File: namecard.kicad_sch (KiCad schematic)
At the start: 37 parts, among them J1 Conn_01x24, J2 Conn_01x05, Q1 AO3400A, U1 STM32G030K6Tx, U2 ST25DV04K-IER8C3

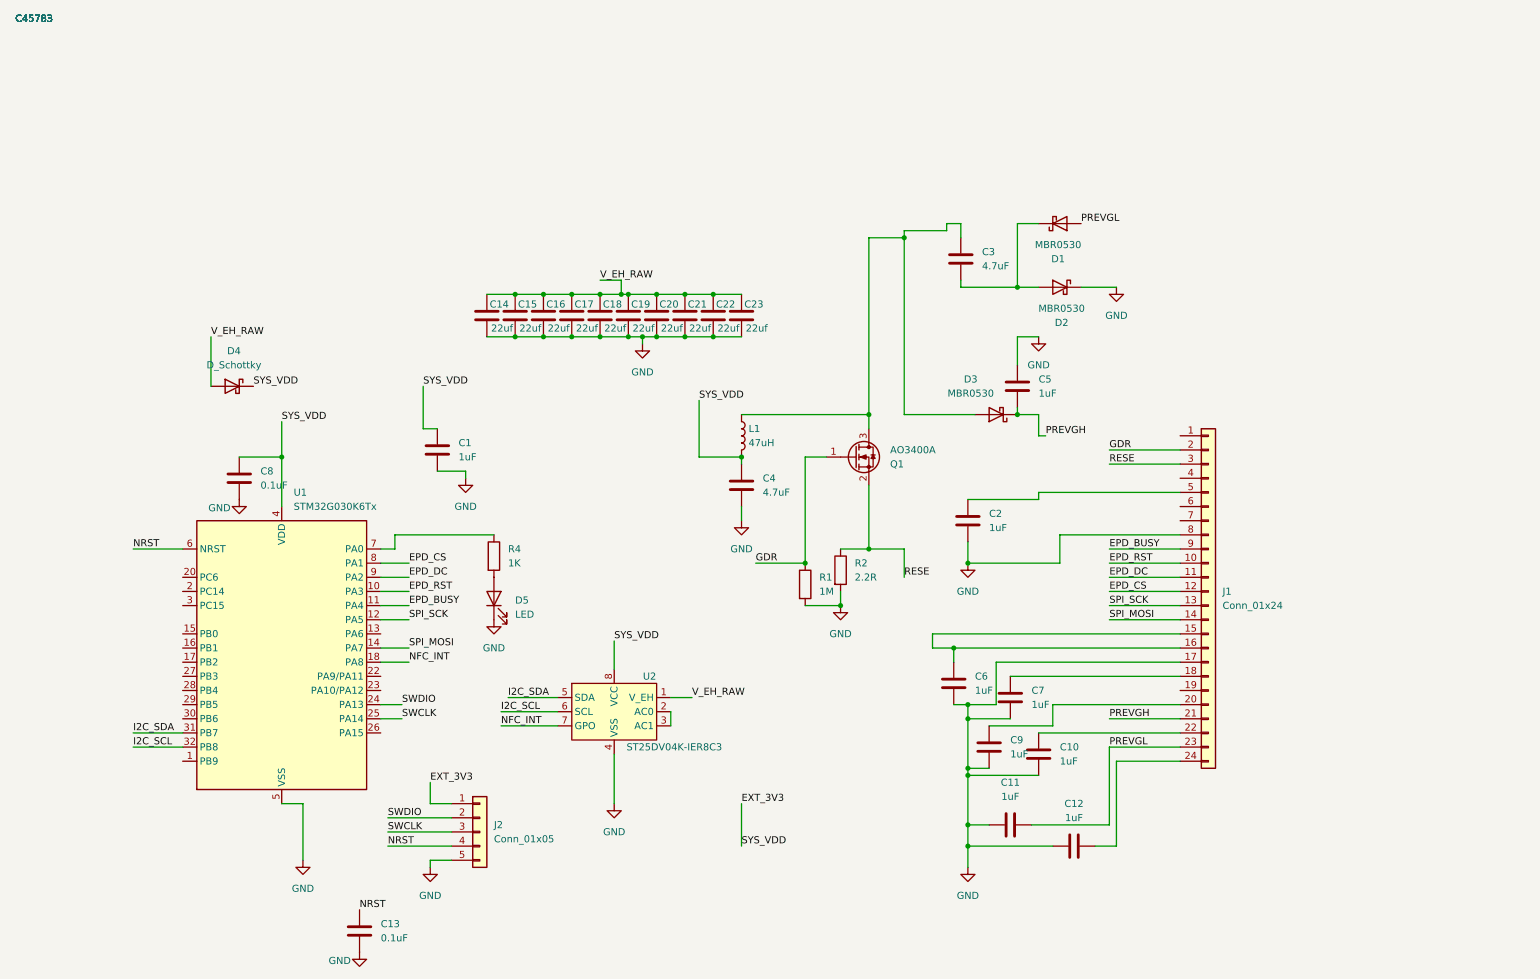
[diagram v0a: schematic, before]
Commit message: v3
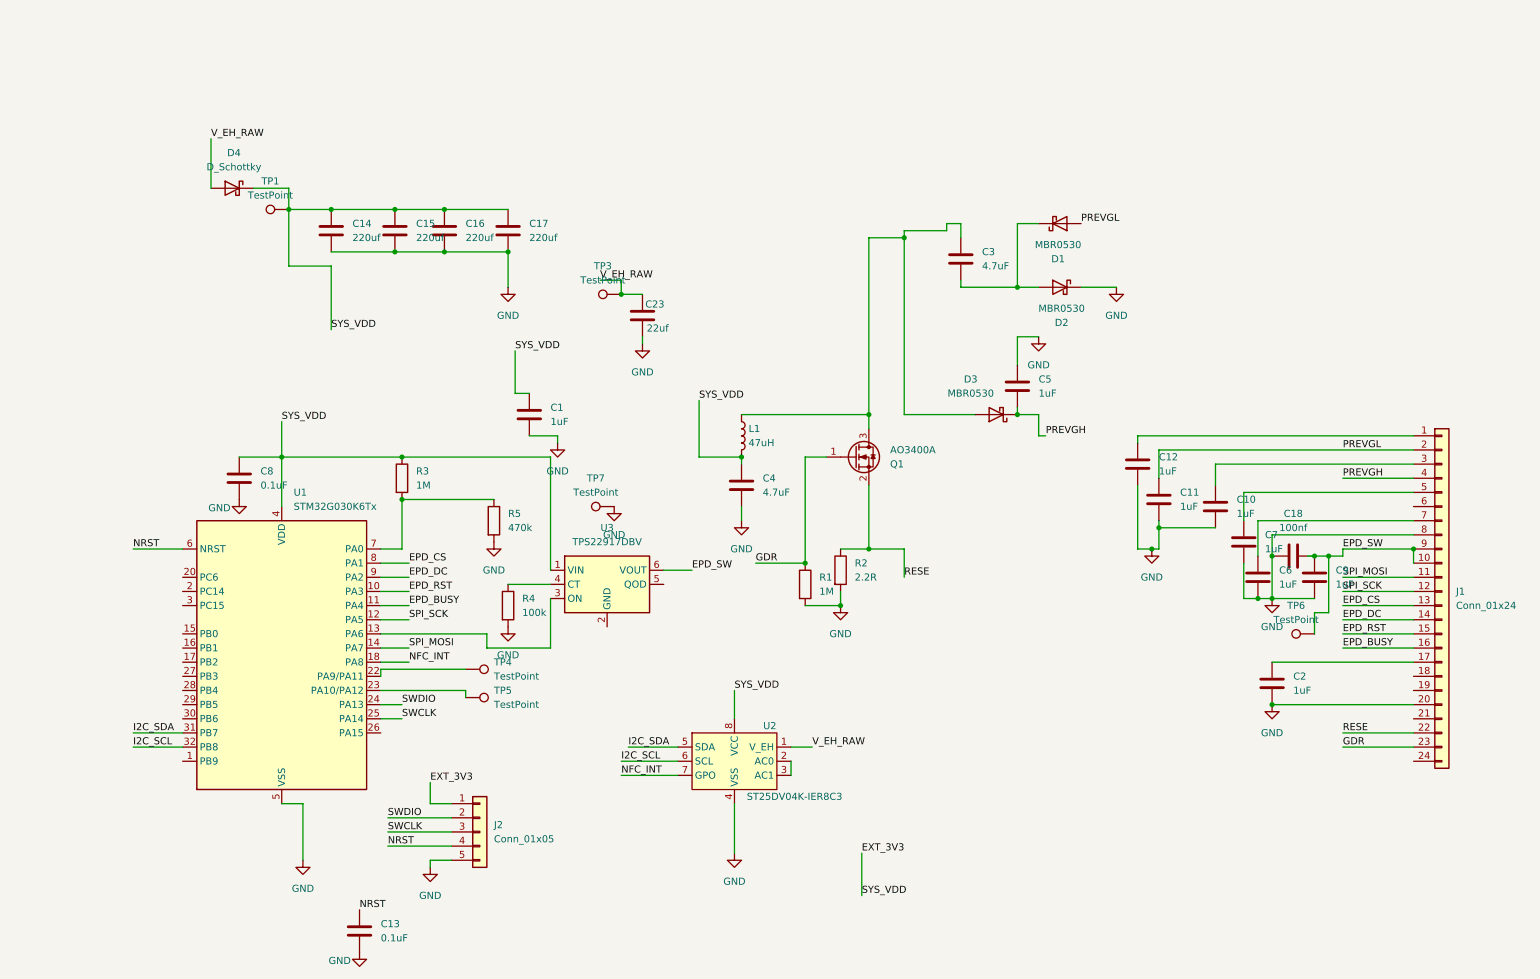
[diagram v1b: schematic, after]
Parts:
- removed C19, C20, C21, C22: 22uf, Capacitor_SMD:C_0805_2012Metric, symbol Device:C
- removed D5: LED, LED_SMD:LED_0603_1608Metric, symbol Device:LED
- added R3: 1M, Resistor_SMD:R_0603_1608Metric, symbol Device:R
- added R5: 470k, Resistor_SMD:R_0603_1608Metric, symbol Device:R
- added TP1, TP3, TP4, TP5, TP6, TP7: TestPoint, TestPoint:TestPoint_Pad_D1.0mm, symbol Connector:TestPoint
- added U3: TPS22917DBV, Package_TO_SOT_SMD:SOT-23-6, symbol Power_Management:TPS22917DBV
- C14, C15, C16, C17: value 22uf -> 220uf; footprint Capacitor_SMD:C_0805_2012Metric -> Capacitor_Tantalum_SMD:6TPE220MAZB; JLCPCB (none) -> C79111; LCSC C45783 -> (none)
- C18: value 22uf -> 100nf; footprint Capacitor_SMD:C_0805_2012Metric -> Capacitor_SMD:C_0603_1608Metric; LCSC C45783 -> (none)
- C23: JLCPCB (none) -> C45783; LCSC C45783 -> (none)
- D4: footprint Diode_SMD:D_SOD-123 -> Diode_SMD:D_SOD-123F; JLCPCB (none) -> C110921; LCSC C22374920 -> (none)
- J1: footprint Connector:FFC-SMD_24P-P0.50_FH34SRJ-24S-0.5SH -> Connector_FFC-FPC:Hirose_FH12-24S-0.5SH_1x24-1MP_P0.50mm_Horizontal; JLCPCB (none) -> C506794; LCSC C324726 -> (none)
- L1: JLCPCB (none) -> C66936; LCSC C66936 -> (none)
- R4: value 1K -> 100k
- U1: JLCPCB (none) -> C529331; LCSC C529331 -> (none)
- U2: JLCPCB (none) -> C2908287; LCSC C2908287 -> (none)
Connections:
- net EPD_BUSY: now also J1.16 (Pin_16); no longer J1.9 (Pin_9)
- net EPD_CS: now also J1.13 (Pin_13); no longer J1.12 (Pin_12)
- net EPD_DC: now also J1.14 (Pin_14); no longer J1.11 (Pin_11)
- net EPD_RST: now also J1.15 (Pin_15); no longer J1.10 (Pin_10)
- net EXT_3V3: now also C14.1, C15.1, C16.1, C17.1, R3.1, TP1.1, U3.1 (VIN)
- net GDR: now also J1.23 (Pin_23); no longer J1.2 (Pin_2)
- net GND: now also C11.2, C18.1, J1.20 (Pin_20), R4.2, R5.2, TP7.1; no longer C11.1, C18.2, J1.17 (Pin_17)
- net PREVGH: now also J1.4 (Pin_4); no longer J1.21 (Pin_21)
- net PREVGL: now also C11.1, J1.2 (Pin_2); no longer C11.2, J1.23 (Pin_23)
- net RESE: now also J1.22 (Pin_22); no longer J1.3 (Pin_3)
- net SPI_MOSI: now also J1.11 (Pin_11); no longer J1.14 (Pin_14)
- net SPI_SCK: now also J1.12 (Pin_12); no longer J1.13 (Pin_13)
- net V_EH_RAW: now also TP3.1; no longer C14.1, C15.1, C16.1, C17.1, C18.1
- net at C7.1: now also J1.5 (Pin_5); no longer J1.18 (Pin_18)
- net at U1.13 (PA6): now also U3.3 (ON)
- net at U1.22 (PA9/PA11): now also TP4.1
- net at U1.23 (PA10/PA12): now also TP5.1
- net at R4.1: now also U3.4 (CT); no longer U1.7 (PA0)
- net at C12.2: now also J1.1 (Pin_1); no longer J1.24 (Pin_24)
- net EPD_SW: now reaches C9.1
- net EPD_SW: now also C18.2, J1.10 (Pin_10), J1.9 (Pin_9), TP6.1, U3.6 (VOUT); no longer J1.20 (Pin_20)
- net at C2.1: now also J1.17 (Pin_17); no longer J1.5 (Pin_5)
- net at C10.1: now also J1.3 (Pin_3); no longer J1.22 (Pin_22)
- net at J1.7 (Pin_7): now also C6.1
- new net: R3.2, R5.1, U1.7 (PA0)
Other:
- moved on the sheet: C1, C10, C11, C12, C2, C23, C6, C7, C9, D4, J1, U2
